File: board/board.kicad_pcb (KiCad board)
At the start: 2 copper layers, 21 x 13 mm, 1 part

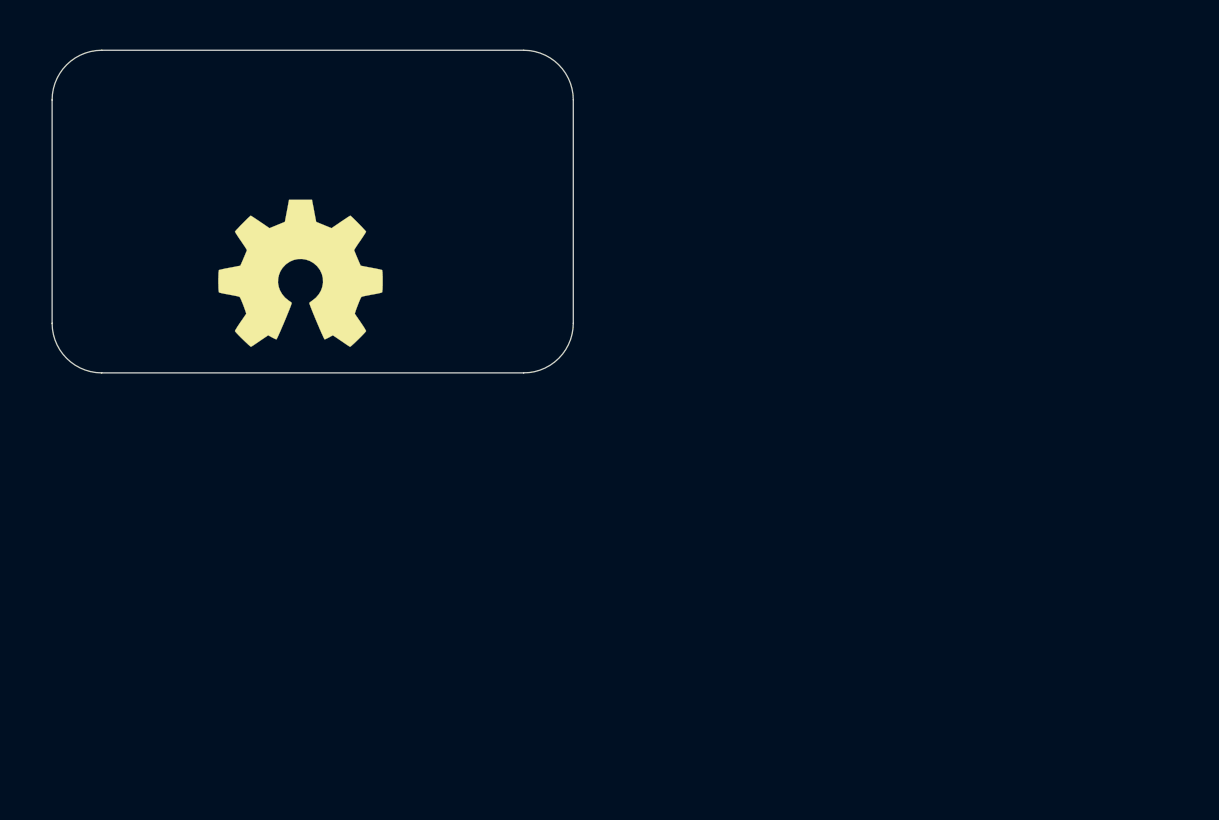
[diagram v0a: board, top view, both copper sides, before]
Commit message: initial
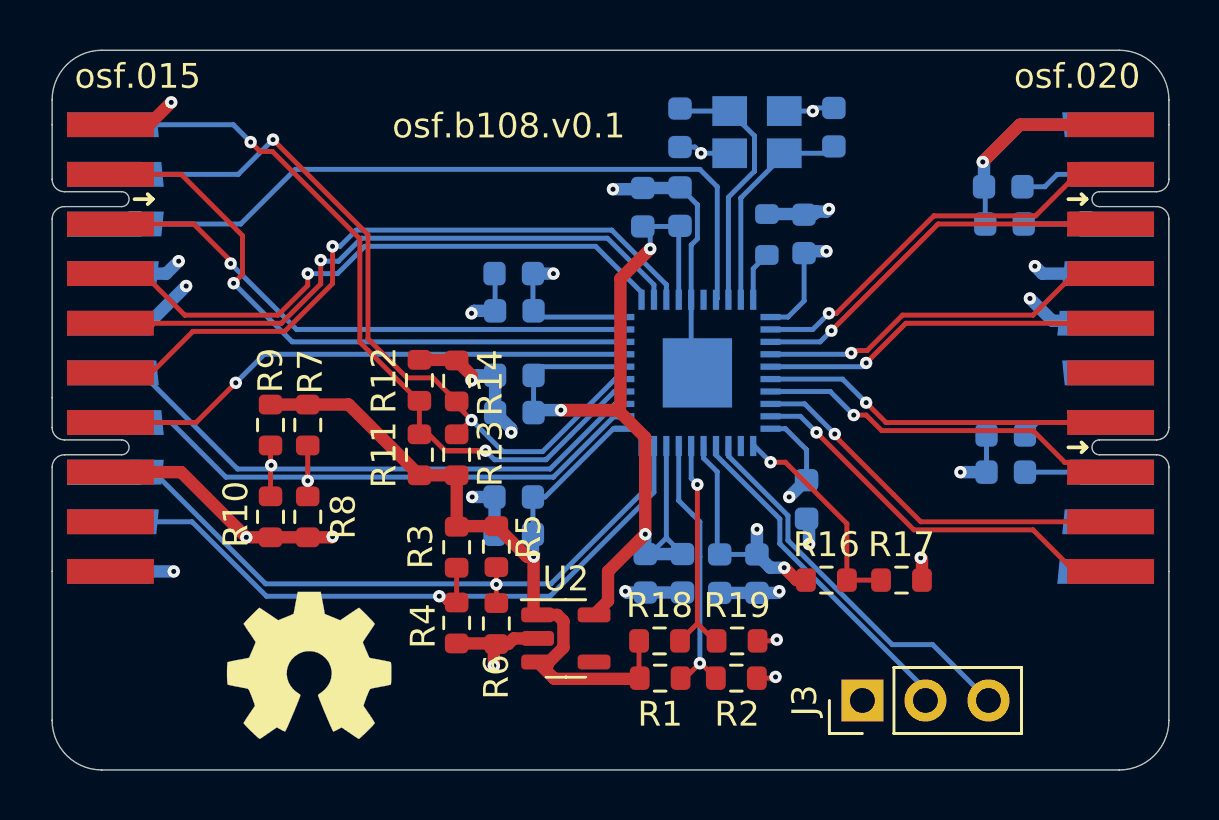
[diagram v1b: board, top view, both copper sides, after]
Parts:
- added C1: 100nF, Capacitor_SMD:C_0603_1608Metric, B.Cu at (178.3, 95.5)
- added C10: 10nF, Capacitor_SMD:C_0603_1608Metric, B.Cu at (158.6, 109.5)
- added C11: 10nF, Capacitor_SMD:C_0603_1608Metric, B.Cu at (166.9, 111.1)
- added C12: 10nF, Capacitor_SMD:C_0603_1608Metric, B.Cu at (158.6, 99.0)
- added C13: 100nF, Capacitor_SMD:C_0603_1608Metric, B.Cu at (170.4, 108.1)
- added C14: 33pF, Capacitor_SMD:C_0603_1608Metric, B.Cu at (165.3, 93.1)
- added C15: 100nF, Capacitor_SMD:C_0603_1608Metric, B.Cu at (170.3, 97.4)
- added C16: 33pF, Capacitor_SMD:C_0603_1608Metric, B.Cu at (171.5, 93.1)
- added C17: 10nF, Capacitor_SMD:C_0603_1608Metric, B.Cu at (158.6, 104.6)
- added C18: 10nF, Capacitor_SMD:C_0603_1608Metric, B.Cu at (165.4, 111.1)
- added C19: 10nF, Capacitor_SMD:C_0603_1608Metric, B.Cu at (158.6, 103.1)
- added C2: 100nF, Capacitor_SMD:C_0603_1608Metric, B.Cu at (178.4, 97.0)
- added C20: 100nF, Capacitor_SMD:C_0603_1608Metric, B.Cu at (163.9, 111.1)
- added C3: 100nF, Capacitor_SMD:C_0603_1608Metric, B.Cu at (178.4, 105.5)
- added C4: 100nF, Capacitor_SMD:C_0603_1608Metric, B.Cu at (178.4, 107.0)
- added C5: 100nF, Capacitor_SMD:C_0603_1608Metric, B.Cu at (165.3, 96.3)
- added C6: 100nF, Capacitor_SMD:C_0603_1608Metric, B.Cu at (163.8, 96.3)
- added C7: 100nF, Capacitor_SMD:C_0603_1608Metric, B.Cu at (158.6, 100.5)
- added C8: 100nF, Capacitor_SMD:C_0603_1608Metric, B.Cu at (158.6, 108.0)
- added C9: 100nF, Capacitor_SMD:C_0603_1608Metric, B.Cu at (168.4, 111.1)
- added J1: 015_RGMII, on_edge:on_edge_2x10_device, F.Cu at (140.0, 97.0)
- added J2: 020_1000BASE-T_with_CT, on_edge:on_edge_2x10_host, F.Cu at (185.0, 97.0)
- added J3: Conn_01x03_Male, Connector_PinHeader_2.54mm:PinHeader_1x03_P2.54mm_Vertical, F.Cu at (172.7, 116.2)
- added R1: 10k, Resistor_SMD:R_0603_1608Metric, F.Cu at (164.5, 115.3)
- added R10: 10k, Resistor_SMD:R_0603_1608Metric, F.Cu at (148.8, 108.8)
- added R11: 10k, Resistor_SMD:R_0603_1608Metric, F.Cu at (154.8, 106.3)
- added R12: 10k, Resistor_SMD:R_0603_1608Metric, F.Cu at (154.8, 103.3)
- added R13: 10k, Resistor_SMD:R_0603_1608Metric, F.Cu at (156.3, 106.3)
- added R14: 10k, Resistor_SMD:R_0603_1608Metric, F.Cu at (156.3, 103.3)
- added R15: 3.01k, Resistor_SMD:R_0603_1608Metric, B.Cu at (168.8, 97.4)
- added R16: 10k, Resistor_SMD:R_0603_1608Metric, F.Cu at (171.2, 111.3)
- added R17: 10k, Resistor_SMD:R_0603_1608Metric, F.Cu at (174.2, 111.3)
- added R18: 10k, Resistor_SMD:R_0603_1608Metric, F.Cu at (164.5, 113.8)
- added R19: 10k, Resistor_SMD:R_0603_1608Metric, F.Cu at (167.6, 113.8)
- added R2: 10k, Resistor_SMD:R_0603_1608Metric, F.Cu at (167.6, 115.3)
- added R3: 10k, Resistor_SMD:R_0603_1608Metric, F.Cu at (156.3, 110.0)
- added R4: 10k, Resistor_SMD:R_0603_1608Metric, F.Cu at (156.3, 113.1)
- added R5: 10k, Resistor_SMD:R_0603_1608Metric, F.Cu at (157.9, 110.0)
- added R6: 10k, Resistor_SMD:R_0603_1608Metric, F.Cu at (157.9, 113.1)
- added R7: 10k, Resistor_SMD:R_0603_1608Metric, F.Cu at (150.3, 105.1)
- added R8: 10k, Resistor_SMD:R_0603_1608Metric, F.Cu at (150.3, 108.8)
- added R9: 10k, Resistor_SMD:R_0603_1608Metric, F.Cu at (148.8, 105.1)
- added U1: , b108:ADIN1300BCPZ, B.Cu at (166.0, 103.0)
- added U2: TLV71209_SOT23-5, Package_TO_SOT_SMD:SOT-23-5, F.Cu at (160.7, 113.7)
- added Y1: Crystal_GND24_Small, Crystal:Crystal_SMD_Abracon_ABM8G-4Pin_3.2x2.5mm, B.Cu at (168.4, 93.3)
- moved LOGO1 15.8 mm to (150.3, 114.8)
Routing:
- net GND: track 0.00 -> 149.6 mm, vias 0 -> 21
- net /ADIN1300/VDD: track 0.00 -> 91.1 mm, vias 0 -> 6
- net +5V: track 0.00 -> 47.9 mm, vias 0 -> 2
- net +3.3V: track 0.00 -> 46.7 mm, vias 0 -> 2
- net /ADIN1300/DVDD: track 0.00 -> 41.2 mm, vias 0 -> 3
- net /ADIN1300/RXC: track 0.00 -> 32.2 mm, vias 0 -> 2
- net /ADIN1300/RX_CTL: track 0.00 -> 31.3 mm, vias 0 -> 2
- net /\reset: track 0.00 -> 30.5 mm
- net /ADIN1300/RXD_3: track 0.00 -> 28.9 mm, vias 0 -> 1
- net /ADIN1300/RXD_2: track 0.00 -> 28.9 mm, vias 0 -> 1
- net /ADIN1300/TXD_3: track 0.00 -> 27.2 mm, vias 0 -> 1
- net /ADIN1300/RXD_0: track 0.00 -> 25.4 mm, vias 0 -> 1
- net /ADIN1300/TXD_2: track 0.00 -> 25.3 mm, vias 0 -> 1
- net /ADIN1300/TXC: track 0.00 -> 25.1 mm, vias 0 -> 1
- net /ADIN1300/RXD_1: track 0.00 -> 24.9 mm, vias 0 -> 1
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- added copper zone on In2.Cu, net GND
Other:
- board size 21 x 13 mm -> 45 x 29 mm
- copper layers 2 -> 4
- board text added: "osf.015"
- board text added: "osf.020"
- board text added: "osf.b108.v0.1"
